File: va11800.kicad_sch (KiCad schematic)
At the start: 265 parts, among them J1 Conn_01x16_Female, J3 Conn_01x16_Female, SW1 RotaryEncoder_Switch, SW2 RotaryEncoder_Switch, SW3 RotaryEncoder_Switch, SW4 RotaryEncoder_Switch, SW5 RotaryEncoder_Switch, j2 MX-NoLED, k1 MX-NoLED, m1 MX-NoLED, p1 MX-NoLED, q1 MX-NoLED, t1 MX-NoLED, u1 MX-NoLED, x1 MX-NoLED, y1 MX-NoLED

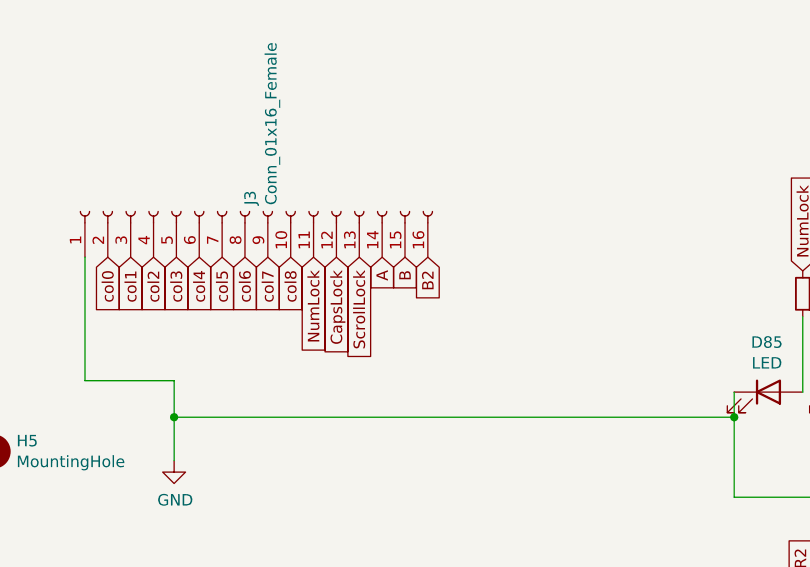
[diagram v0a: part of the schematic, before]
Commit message: cleanup traces
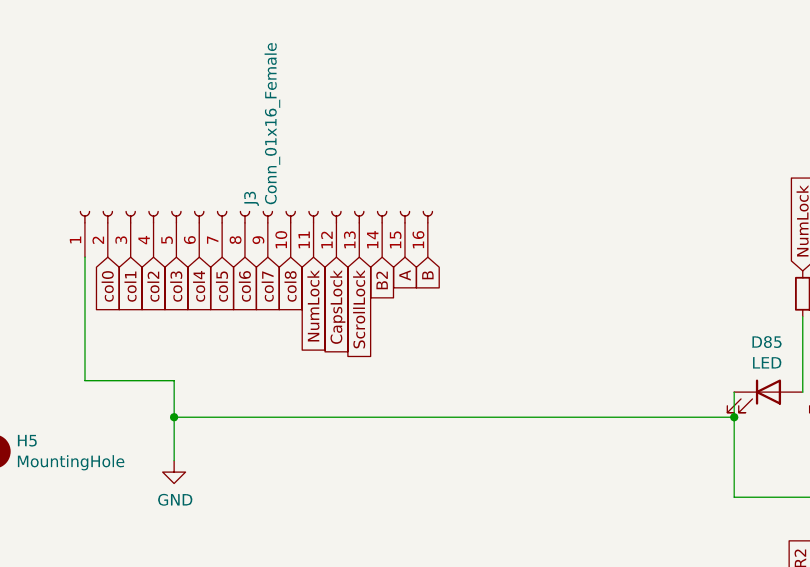
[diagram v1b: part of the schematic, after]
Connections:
- net A: now also J3.15 (Pin_15); no longer J3.14 (Pin_14)
- net B: now also J3.16 (Pin_16); no longer J3.15 (Pin_15)
- net B2: now also J3.14 (Pin_14); no longer J3.16 (Pin_16)
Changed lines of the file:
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@@
     )
   )
-  (global_label "B" (shape input) (at 343.408 137.414 270) (fields_autoplaced)
-    (effects (font (size 1.27 1.27)) (justify right))
-    (property "Intersheet References" "${INTERSHEET_REFS}" (id 0) (at 343.3286 141.0082 90)
+  (global_label "B" (shape input) (at 345.948 137.414 270) (fields_autoplaced)
+    (effects (font (size 1.27 1.27)) (justify right))
+    (property "Intersheet References" "${INTERSHEET_REFS}" (id 0) (at 345.8686 141.0082 90)
       (effects (font (size 1.27 1.27)) (justify right) hide)
     )
@@
     )
   )
-  (global_label "A" (shape input) (at 340.868 137.414 270) (fields_autoplaced)
-    (effects (font (size 1.27 1.27)) (justify right))
-    (property "Intersheet References" "${INTERSHEET_REFS}" (id 0) (at 340.7886 140.8268 90)
+  (global_label "A" (shape input) (at 343.408 137.414 270) (fields_autoplaced)
+    (effects (font (size 1.27 1.27)) (justify right))
+    (property "Intersheet References" "${INTERSHEET_REFS}" (id 0) (at 343.3286 140.8268 90)
       (effects (font (size 1.27 1.27)) (justify right) hide)
     )
@@
     )
   )
-  (global_label "B2" (shape input) (at 345.948 137.414 270) (fields_autoplaced)
-    (effects (font (size 1.27 1.27)) (justify right))
-    (property "Intersheet References" "${INTERSHEET_REFS}" (id 0) (at 345.8686 142.2177 90)
-      (effects (font (size 1.27 1.27)) (justify right) hide)
-    )
+  (global_label "B2" (shape input) (at 340.868 137.414 270) (fields_autoplaced)
+    (effects (font (size 1.27 1.27)) (justify right))
+    (property "Intersheet References" "${INTERSHEET_REFS}" (id 0) (at 340.7886 142.2177 90)
+      (effects (font (size 1.27 1.27)) (justify right) hide)
+    )
